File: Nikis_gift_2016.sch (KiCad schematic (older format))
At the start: 32 parts, among them CON1 BARREL_JACK, IC1 ATMEGA328P-A, P1 CONN_01X06, SW1 SW_PUSH, SW2 SW_PUSH, SW3 SW_PUSH, SW4 SW_PUSH, SW5 SW_PUSH, U1 LM7805CT, U2 DS1338

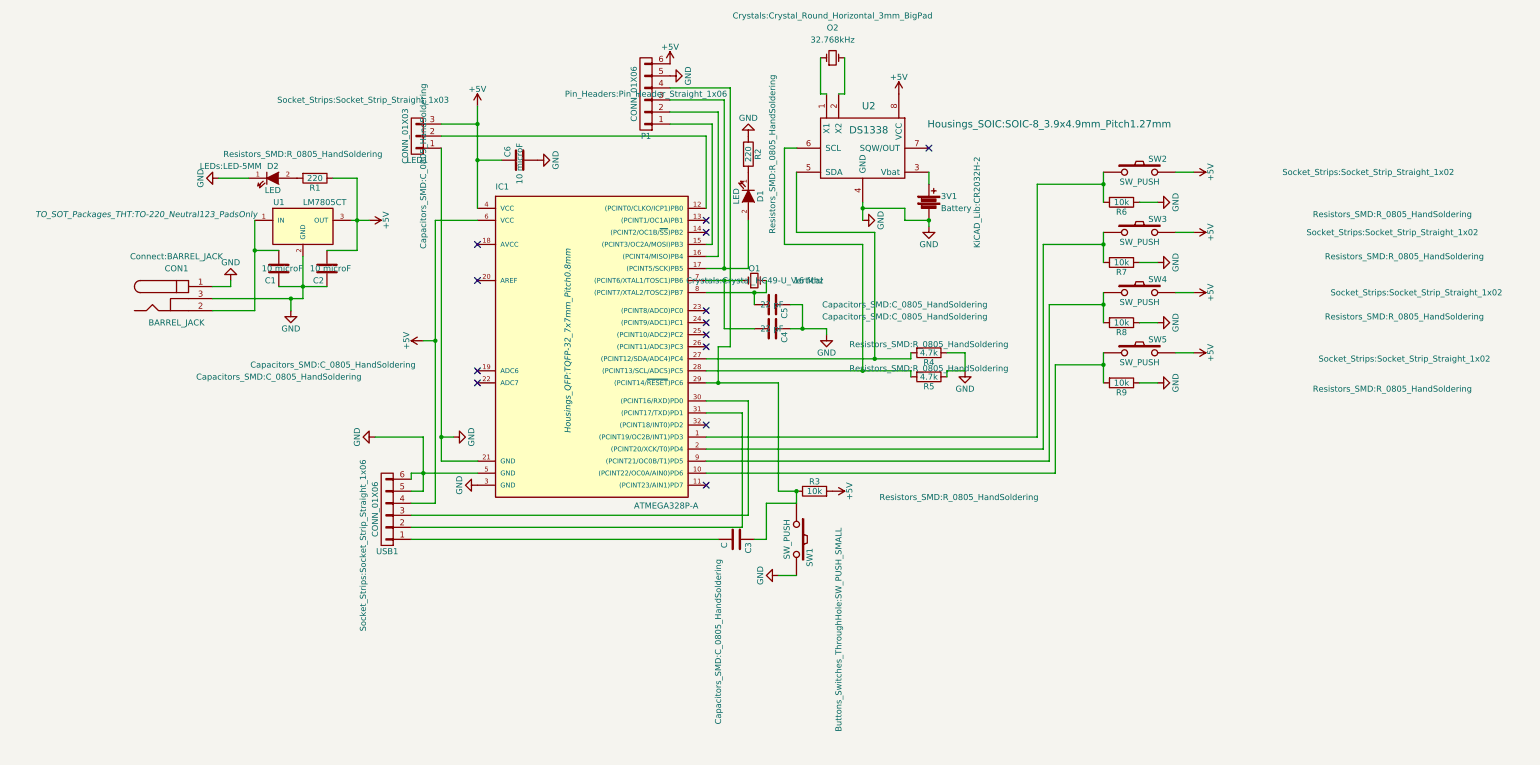
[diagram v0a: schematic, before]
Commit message: gerber
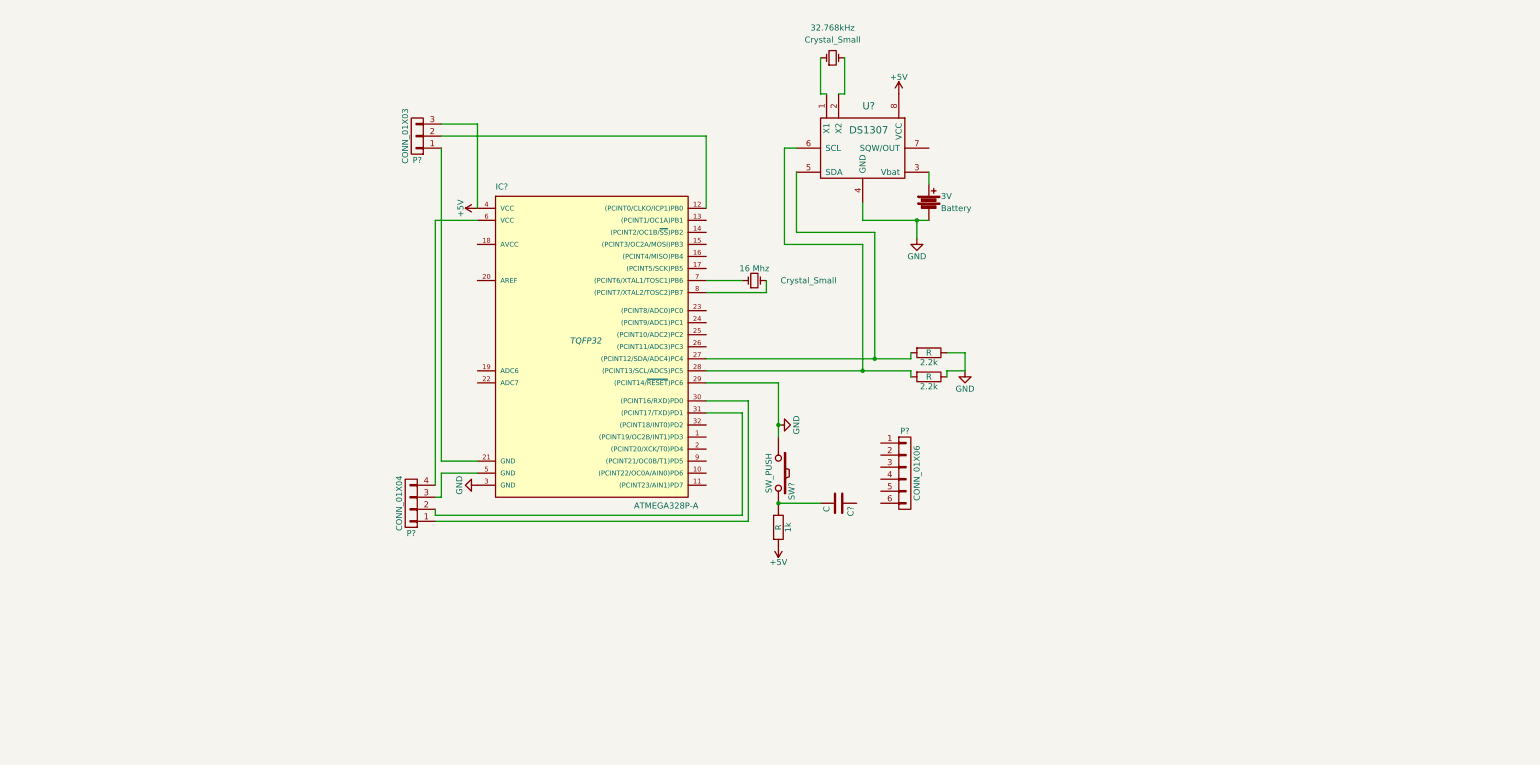
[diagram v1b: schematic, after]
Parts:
- removed C1, C2, C6: 10 microF, Capacitors_SMD:C_0805_HandSoldering, symbol C
- removed C4, C5: 22 pF, Capacitors_SMD:C_0805_HandSoldering, symbol C
- removed CON1: BARREL_JACK, Connect:BARREL_JACK, symbol BARREL_JACK
- removed D1, D2: LED, LEDs:LED-5MM, symbol LED
- removed P1: CONN_01X06, Pin_Headers:Pin_Header_Straight_1x06, symbol CONN_01X06
- removed R1, R2: 220, Resistors_SMD:R_0805_HandSoldering, symbol R
- removed R6, R7, R8, R9: 10k, Resistors_SMD:R_0805_HandSoldering, symbol R
- removed SW2, SW3, SW4, SW5: SW_PUSH, Socket_Strips:Socket_Strip_Straight_1x02, symbol SW_PUSH
- removed U1: LM7805CT, TO_SOT_Packages_THT:TO-220_Neutral123_PadsOnly, symbol LM7805CT
- added P?: CONN_01X04, symbol CONN_01X04
- 16~Mhz: renamed from O1; value 16 Mhz -> Crystal_Small; footprint Crystals:Crystal_HC49-U_Vertical -> (none)
- 1k: renamed from R3; value 10k -> R; footprint Resistors_SMD:R_0805_HandSoldering -> (none)
- 2.2k: renamed from R4; value 4.7k -> R; footprint Resistors_SMD:R_0805_HandSoldering -> (none)
- 2.2k: renamed from R5; value 4.7k -> R; footprint Resistors_SMD:R_0805_HandSoldering -> (none)
- 32.768kHz: renamed from O2; value 32.768kHz -> Crystal_Small; footprint Crystals:Crystal_Round_Horizontal_3mm_BigPad -> (none)
- 3V: renamed from 3V1; footprint KiCAD_Lib:CR2032H-2 -> (none)
- C?: renamed from C3; footprint Capacitors_SMD:C_0805_HandSoldering -> (none)
- IC?: renamed from IC1; footprint Housings_QFP:TQFP-32_7x7mm_Pitch0.8mm -> TQFP32
- P?: renamed from LED1; footprint Socket_Strips:Socket_Strip_Straight_1x03 -> (none)
- P?: renamed from USB1; footprint Socket_Strips:Socket_Strip_Straight_1x06 -> (none)
- SW?: renamed from SW1; footprint Buttons_Switches_ThroughHole:SW_PUSH_SMALL -> (none)
- U?: renamed from U2; value DS1338 -> DS1307; footprint Housings_SOIC:SOIC-8_3.9x4.9mm_Pitch1.27mm -> (none)
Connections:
- net +5V: no longer IC?.6 (VCC), P?.4 (P4)
- net GND: now also IC?.29 ((PCINT14/~RESET~)PC6), SW?.1; no longer IC?.21 (GND), IC?.5 (GND), P?.1 (P1), P?.5 (P5), P?.6 (P6), SW?.2
- net at IC?.30 ((PCINT16/RXD)PD0): now also P?.1 (P1); no longer P?.3 (P3)
- net at IC?.31 ((PCINT17/TXD)PD1): now also P?.2 (P2); no longer P?.2 (P2)
- net at C?.2: no longer P?.1 (P1)
- new net: IC?.21 (GND), P?.1 (P1)
- new net: IC?.5 (GND), P?.3 (P3)
- new net: IC?.6 (VCC), P?.4 (P4)
- new net: 1k.1, SW?.2
- now unconnected: C?.1
- no-connect marks 13 -> 0
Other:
- moved on the sheet: 1k, C?, P?, SW?

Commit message: updating layout and schematic
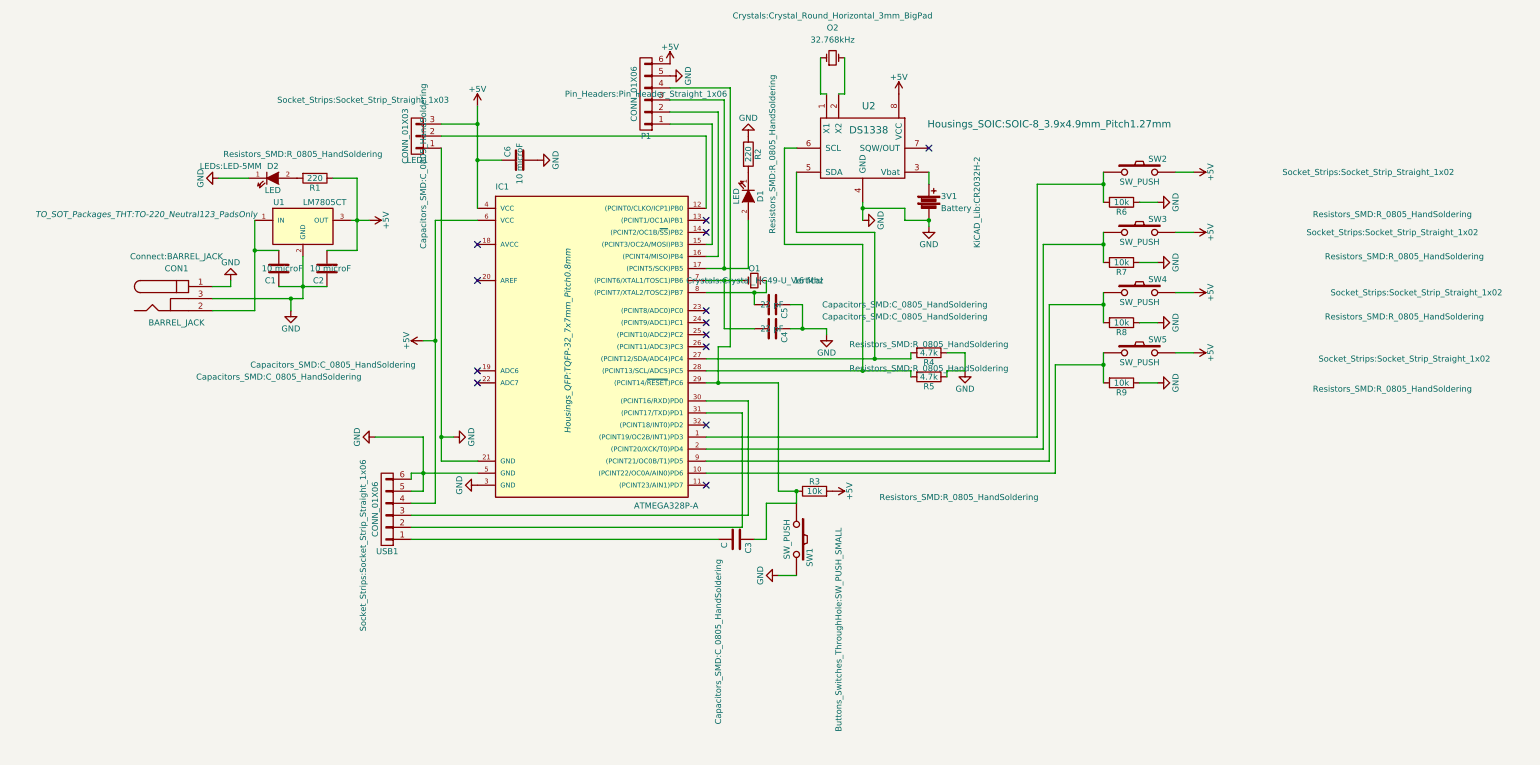
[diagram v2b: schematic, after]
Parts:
- removed P?: CONN_01X04, symbol CONN_01X04
- added C1, C2, C6: 10 microF, Capacitors_SMD:C_0805_HandSoldering, symbol C
- added C4, C5: 22 pF, Capacitors_SMD:C_0805_HandSoldering, symbol C
- added CON1: BARREL_JACK, Connect:BARREL_JACK, symbol BARREL_JACK
- added D1, D2: LED, LEDs:LED-5MM, symbol LED
- added P1: CONN_01X06, Pin_Headers:Pin_Header_Straight_1x06, symbol CONN_01X06
- added R1, R2: 220, Resistors_SMD:R_0805_HandSoldering, symbol R
- added R6, R7, R8, R9: 10k, Resistors_SMD:R_0805_HandSoldering, symbol R
- added SW2, SW3, SW4, SW5: SW_PUSH, Socket_Strips:Socket_Strip_Straight_1x02, symbol SW_PUSH
- added U1: LM7805CT, TO_SOT_Packages_THT:TO-220_Neutral123_PadsOnly, symbol LM7805CT
- 3V1: renamed from 3V; footprint (none) -> KiCAD_Lib:CR2032H-2
- C3: renamed from C?; footprint (none) -> Capacitors_SMD:C_0805_HandSoldering
- IC1: renamed from IC?; footprint TQFP32 -> Housings_QFP:TQFP-32_7x7mm_Pitch0.8mm
- LED1: renamed from P?; footprint (none) -> Socket_Strips:Socket_Strip_Straight_1x03
- O1: renamed from 16~Mhz; value Crystal_Small -> 16 Mhz; footprint (none) -> Crystals:Crystal_HC49-U_Vertical
- O2: renamed from 32.768kHz; value Crystal_Small -> 32.768kHz; footprint (none) -> Crystals:Crystal_Round_Horizontal_3mm_BigPad
- R3: renamed from 1k; value R -> 10k; footprint (none) -> Resistors_SMD:R_0805_HandSoldering
- R4, R5: renamed from 2.2k; value R -> 4.7k; footprint (none) -> Resistors_SMD:R_0805_HandSoldering
- SW1: renamed from SW?; footprint (none) -> Buttons_Switches_ThroughHole:SW_PUSH_SMALL
- U2: renamed from U?; value DS1307 -> DS1338; footprint (none) -> Housings_SOIC:SOIC-8_3.9x4.9mm_Pitch1.27mm
- USB1: renamed from P?; footprint (none) -> Socket_Strips:Socket_Strip_Straight_1x06
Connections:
- net +5V: now also IC1.6 (VCC), USB1.4 (P4), C2.2, C6.1, P1.6 (P6), R1.1, SW2.2, SW3.2, SW4.2, SW5.2, U1.3 (OUT)
- net GND: now also IC1.21 (GND), IC1.5 (GND), LED1.1 (P1), SW1.2, USB1.5 (P5), USB1.6 (P6), C1.1, C2.1, C4.1, C5.1, C6.2, CON1.1, CON1.3, D2.1 (K), P1.5 (P5), R2.1, R6.1, R7.1, R8.1, R9.1, U1.2 (GND); no longer IC1.29 ((PCINT14/~RESET~)PC6), SW1.1
- net at IC1.1 ((PCINT19/OC2B/INT1)PD3): now also R6.2, SW2.1
- net at IC1.10 ((PCINT22/OC0A/AIN0)PD6): now also R9.2, SW5.1
- net at IC1.15 ((PCINT3/OC2A/MOSI)PB3): now also P1.1 (P1)
- net at IC1.16 ((PCINT4/MISO)PB4): now also P1.2 (P2)
- net at IC1.17 ((PCINT5/SCK)PB5): now also D1.2 (A), P1.3 (P3)
- net at IC1.2 ((PCINT20/XCK/T0)PD4): now also R7.2, SW3.1
- net at IC1.30 ((PCINT16/RXD)PD0): now also USB1.3 (P3)
- net at IC1.31 ((PCINT17/TXD)PD1): now also USB1.2 (P2)
- net at IC1.7 ((PCINT6/XTAL1/TOSC1)PB6), O1.1: now also C4.2
- net at IC1.8 ((PCINT7/XTAL2/TOSC2)PB7), O1.2: now also C5.2
- net at IC1.9 ((PCINT21/OC0B/T1)PD5): now also R8.2, SW4.1
- net at R3.1: now also C3.1, IC1.29 ((PCINT14/~RESET~)PC6), SW1.1, P1.4 (P4); no longer SW1.2
- net at C3.2: now also USB1.1 (P1)
- new net: D1.1 (K), R2.2
- new net: C1.2, CON1.2, U1.1 (IN)
- new net: D2.2 (A), R1.2
- no-connect marks 0 -> 13
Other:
- moved on the sheet: C3, R3, SW1, USB1
